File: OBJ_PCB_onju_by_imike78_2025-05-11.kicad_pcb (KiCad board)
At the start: 4 copper layers, 74.5 x 70.6 mm, 177 parts, among them J1 1775443-2, J2 TE_2345986-1, Q1 LBSS138WT1G, Q2 BC847B, SW1 CHS-01TA, U1 TPS62130, U10 SN74LVC125APWR, U11 MAX98357AETE_T, U12 FSUSB42MUX, U13 AP22802AW5-7, U2 MIC5365-1.8YC5-TR, U3 TPS62130, U4 MIC5365-0.9YC5-TR, U5 ESP32-S3R8, U6 W25Q128JVSIQ, U7 XU316-1024-QF60B-C24, U8 W25Q128JVSIQ, U9 TLV73333PDBVR, Y1 40MHz, Y2 24MHz

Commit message: production preparation
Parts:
- J2: value TE_2345986-1 -> usb_c
- R44, R7: value 49.9 -> 49.9R
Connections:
- J2 pad SH1: (no net) -> GND
- J2 pad SH2: (no net) -> GND
- J2 pad SH3: (no net) -> GND
- J2 pad SH4: (no net) -> GND
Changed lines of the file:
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@@
 		)
 		(pad_to_mask_clearance 0.03)
-		(solder_mask_min_width 0.07)
 		(allow_soldermask_bridges_in_footprints yes)
 		(tenting front back)
@@
 			)
 		)
-		(property "Value" "49.9"
+		(property "Value" "49.9R"
 			(at 0 1.43 0)
 			(layer "F.Fab")
@@
 			)
 		)
-		(property "Value" "49.9"
+		(property "Value" "49.9R"
 			(at 0 1.43 0)
 			(layer "F.Fab")
@@
 			)
 		)
-		(property "Value" "TE_2345986-1"
+		(property "Value" "usb_c"
 			(at 2.52 -6.085 37)
 			(layer "F.Fab")
@@
 			(layers "*.Cu")
 			(remove_unused_layers no)
+			(net 1 "GND")
+			(pinfunction "SHIELD")
+			(pintype "passive")
 			(thermal_bridge_angle 90)
 			(options
@@
 			(layers "*.Cu")
 			(remove_unused_layers no)
+			(net 1 "GND")
+			(pinfunction "SHIELD")
+			(pintype "passive")
 			(thermal_bridge_angle 90)
 			(options
@@
 			(layers "*.Cu" "*.Mask")
 			(remove_unused_layers no)
+			(net 1 "GND")
+			(pinfunction "SHIELD")
+			(pintype "passive")
 			(solder_mask_margin 0.102)
 		)
@@
 			(layers "*.Cu" "*.Mask")
 			(remove_unused_layers no)
+			(net 1 "GND")
+			(pinfunction "SHIELD")
+			(pintype "passive")
 			(solder_mask_margin 0.102)
 		)

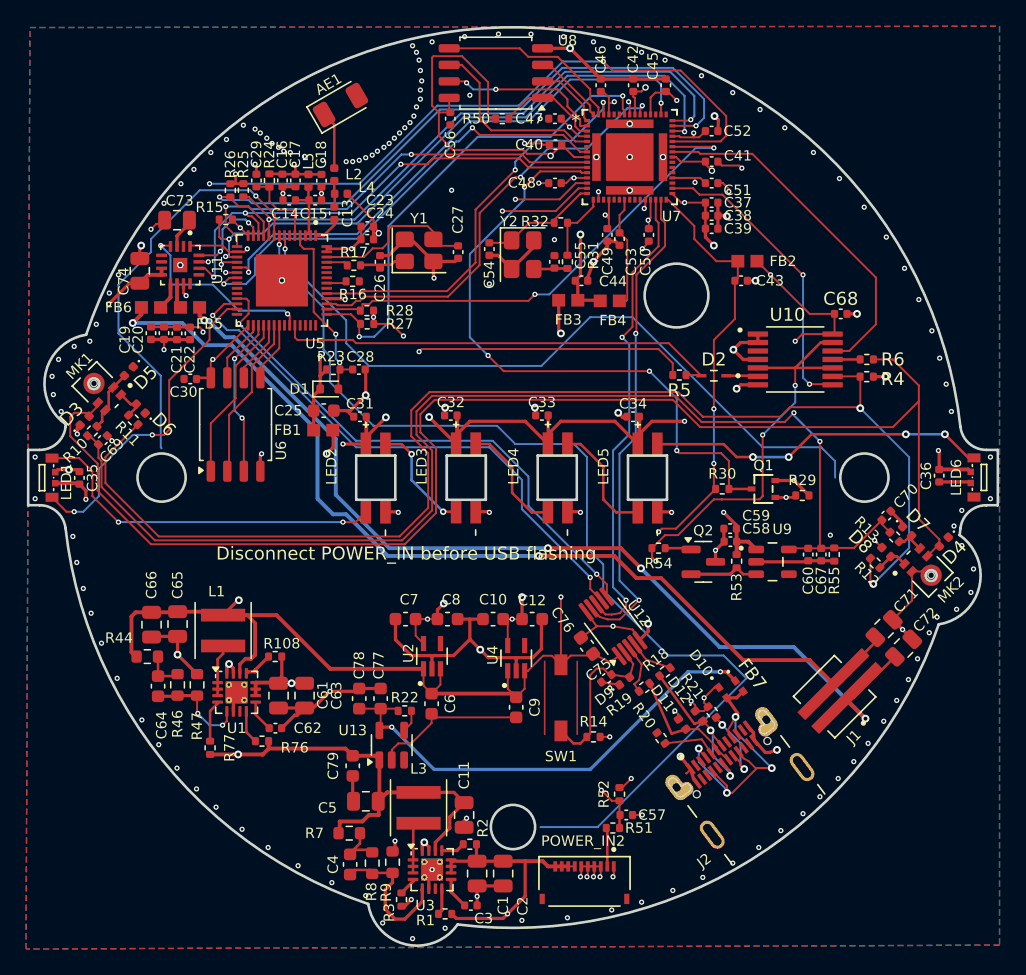
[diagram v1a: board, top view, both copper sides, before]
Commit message: final touches
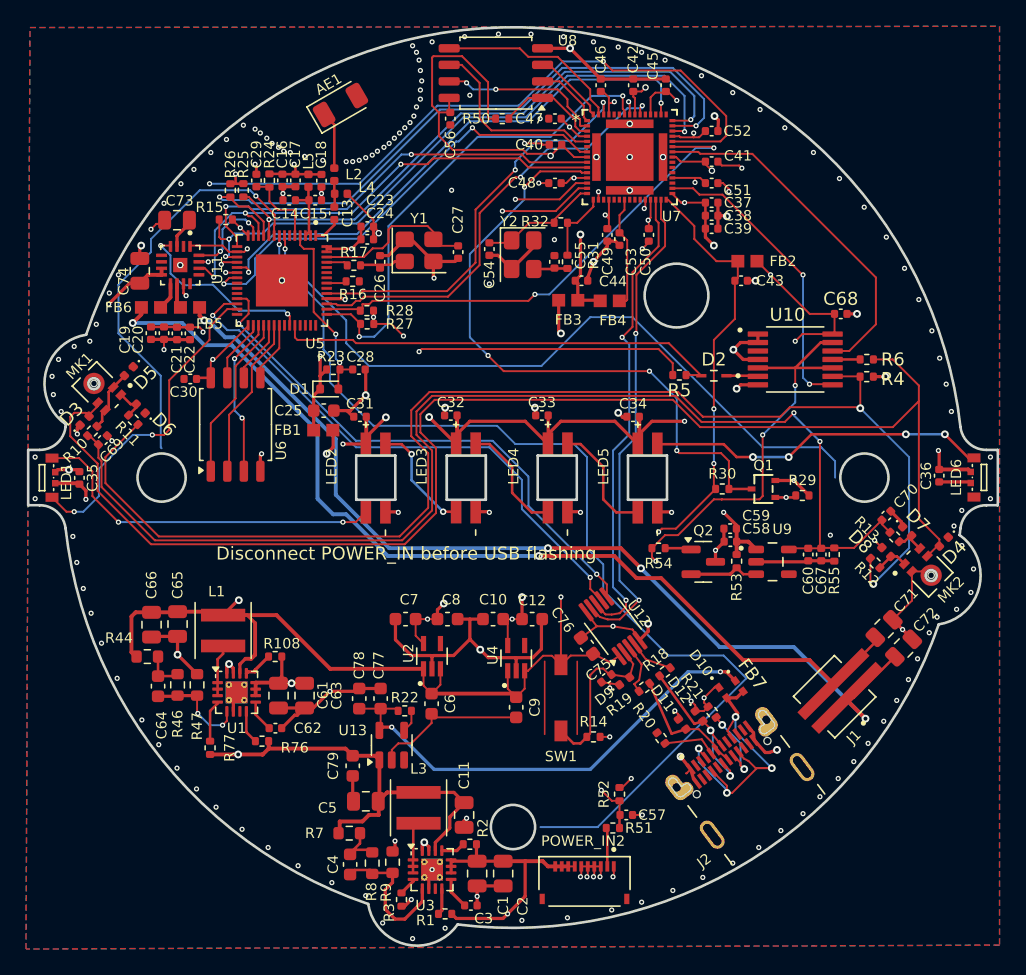
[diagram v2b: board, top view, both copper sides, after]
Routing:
- net GND: track 203.4 -> 202.8 mm
- net AUDIO_PA_EN: track 15.0 -> 14.5 mm
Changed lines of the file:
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@@
 	)
 	(segment
-		(start 154.344033 109.344033)
-		(end 154.344033 109.239039)
-		(width 0.15)
-		(layer "F.Cu")
-		(net 1)
-	)
-	(segment
 		(start 152.75 79.25)
 		(end 153.5 80)
@@
 	)
 	(segment
-		(start 102.557053 85.042947)
-		(end 102.457053 85.042947)
-		(width 0.15)
-		(layer "F.Cu")
-		(net 1)
-	)
-	(segment
 		(start 151.638907 105.201364)
 		(end 151.298636 105.201364)
@@
 	)
 	(segment
-		(start 102.771159 85.042947)
-		(end 102.814106 85)
-		(width 0.15)
-		(layer "F.Cu")
-		(net 1)
-	)
-	(segment
 		(start 109 78.46)
 		(end 109 79.25)
@@
 	)
 	(segment
-		(start 102.557053 85.042947)
-		(end 102.657053 84.942947)
-		(width 0.15)
-		(layer "F.Cu")
-		(net 1)
-	)
-	(segment
 		(start 125.100362 69.285999)
 		(end 125.100362 69.790999)
@@
 	)
 	(segment
-		(start 102.557053 85.042947)
-		(end 102.771159 85.042947)
-		(width 0.15)
-		(layer "F.Cu")
-		(net 1)
-	)
-	(segment
 		(start 148.52812 107.632662)
 		(end 148.52812 107.27812)
@@
 	)
 	(segment
+		(start 109.5 83.5)
+		(end 109 84)
+		(width 0.25)
+		(layer "In2.Cu")
+		(net 4)
+	)
+	(segment
 		(start 118.8 104.88)
 		(end 118.8 106.25)
@@
 	)
 	(segment
-		(start 109 80)
-		(end 108.25 80)
+		(start 108.25 80)
+		(end 109 80.8)
 		(width 0.25)
 		(layer "In2.Cu")
@@
 	)
 	(segment
-		(start 109 84)
-		(end 109 83.5)
-		(width 0.25)
-		(layer "In2.Cu")
-		(net 4)
-	)
-	(segment
 		(start 104.75 102.75)
 		(end 104.75 92.5)
@@
 	)
 	(segment
+		(start 116 83.5)
+		(end 109.5 83.5)
+		(width 0.25)
+		(layer "In2.Cu")
+		(net 4)
+	)
+	(segment
 		(start 126.05 84.45)
 		(end 126.8 83.7)
@@
 	)
 	(segment
-		(start 109 83.5)
-		(end 116 83.5)
-		(width 0.25)
-		(layer "In2.Cu")
-		(net 4)
-	)
-	(segment
-		(start 109 83.5)
-		(end 109 80)
+		(start 128.5 83.7)
+		(end 129.227091 84.427091)
 		(width 0.25)
 		(layer "In2.Cu")
@@
 	)
 	(segment
-		(start 128.5 83.7)
-		(end 129.227091 84.427091)
+		(start 106.25 104.25)
+		(end 104.75 102.75)
 		(width 0.25)
 		(layer "In2.Cu")
@@
 	)
 	(segment
-		(start 106.25 104.25)
-		(end 104.75 102.75)
+		(start 109 80.8)
+		(end 109 84)
 		(width 0.25)
 		(layer "In2.Cu")
@@
 	)
 	(segment
-		(start 128.761361 120.75)
-		(end 128.847862 120.663499)
-		(width 0.2)
-		(layer "F.Cu")
-		(net 16)
-	)
-	(segment
 		(start 126.75 123)
 		(end 127.5 123)
@@
 	)
 	(segment
-		(start 142.4 67.1)
-		(end 142.385113 67.114887)
-		(width 0.15)
-		(layer "F.Cu")
-		(net 22)
-	)
-	(segment
 		(start 145.985563 67.725999)
 		(end 145.985563 68.314437)
@@
 	)
 	(segment
-		(start 136.5 98.25)
-		(end 136.510362 98.260362)
-		(width 0.25)
-		(layer "F.Cu")
-		(net 23)
-	)
-	(segment
 		(start 135.060362 99.950999)
 		(end 135.410362 100.300999)
@@
 	)
 	(segment
-		(start 118.100362 65.765)
-		(end 117.729001 65.765)
-		(width 0.2)
-		(layer "F.Cu")
-		(net 28)
-	)
-	(segment
 		(start 112.595 80.155)
 		(end 112.75 80)
@@
 	)
 	(segment
-		(start 114.862182 69.887818)
-		(end 114.904534 69.93017)
-		(width 0.15)
-		(layer "B.Cu")
-		(net 35)
-	)
-	(segment
 		(start 134.5 69.1)
 		(end 119.3 69.1)
@@
 	)
 	(segment
-		(start 114.85 69.9)
-		(end 114.862182 69.887818)
-		(width 0.15)
-		(layer "In2.Cu")
-		(net 35)
-	)
-	(segment
 		(start 136.5 64.25)
 		(end 137.101049 64.851049)
@@
 	)
 	(segment
-		(start 149.416157 61.640735)
-		(end 149.479039 61.577853)
-		(width 0.15)
-		(layer "B.Cu")
-		(net 52)
-	)
-	(segment
 		(start 117.067099 69.249006)
 		(end 123.650994 69.249006)
@@
 	)
 	(segment
-		(start 113.25 67.5)
-		(end 113.27 67.52)
-		(width 0.15)
-		(layer "F.Cu")
-		(net 53)
-	)
-	(segment
 		(start 116.660362 69.410362)
 		(end 115.5 68.25)
@@
 	)
 	(segment
-		(start 114.100362 67.52)
-		(end 114.25 67.669638)
-		(width 0.15)
-		(layer "F.Cu")
-		(net 53)
-	)
-	(segment
 		(start 115.5 68.25)
 		(end 114.75 68.25)
@@
 	)
 	(segment
-		(start 109.5 74.25)
-		(end 109.5 72)
+		(start 110.5 74.3)
+		(end 109.5 73.4)
 		(width 0.15)
 		(layer "B.Cu")
@@
 	)
 	(segment
+		(start 109.5 73.4)
+		(end 109.5 72)
+		(width 0.15)
+		(layer "B.Cu")
+		(net 65)
+	)
+	(segment
 		(start 114.75 76.25)
 		(end 112.75 74.25)
@@
 	(segment
 		(start 112.75 74.25)
-		(end 109.5 74.25)
+		(end 110.5 74.3)
 		(width 0.15)
 		(layer "B.Cu")
@@
 	)
 	(segment
-		(start 124.5 86.25)
-		(end 134.25 86.25)
-		(width 0.15)
-		(layer "B.Cu")
-		(net 75)
-	)
-	(segment
 		(start 137 89)
 		(end 137 91.25)
@@
 	(segment
 		(start 123.75 86.25)
-		(end 124.5 86.25)
+		(end 134.25 86.25)
 		(width 0.15)
 		(layer "B.Cu")
@@
 	)
 	(segment
-		(start 139.560362 63.5)
-		(end 139.689221 63.5)
-		(width 0.2)
-		(layer "F.Cu")
-		(net 91)
-	)
-	(segment
 		(start 131.9 56.7)
 		(end 133.9 58.7)
@@
 	)
 	(segment
-		(start 147.25 69.25)
-		(end 147.5 69.5)
-		(width 0.15)
-		(layer "F.Cu")
-		(net 115)
-	)
-	(segment
 		(start 147.5 69.5)
 		(end 147.5 71.3)
@@
 	(segment
 		(start 147.185713 69.185713)
-		(end 147.25 69.25)
+		(end 147.5 69.5)
 		(width 0.15)
 		(layer "F.Cu")
@@
 		(net 118)
 	)
-	(segment
-		(start 103.129376 85.860624)
-		(end 103.129376 86.089376)
-		(width 0.2)
-		(layer "F.Cu")
-		(net 118)
-	)
 	(via
 		(at 159.4 86.3)
@@
 	)
 	(segment
-		(start 145.7 96.8)
+		(start 145.3 96.8)
 		(end 147.2 96.8)
 		(width 0.3)
@@
 		(net 132)
 	)
-	(segment
-		(start 145.3 96.8)
-		(end 145.7 96.8)
-		(width 0.3)
-		(layer "F.Cu")
-		(net 132)
-	)
 	(via
 		(at 137.8 95.1)
@@
 	)
 	(segment
-		(start 161.4 106)
-		(end 161.5 106)
-		(width 0.15)
-		(layer "F.Cu")
-		(net 133)
-	)
-	(segment
 		(start 161.5 106.2)
 		(end 161.5 106)
@@
 	(segment
 		(start 151.7 102.1)
-		(end 152.9 102.1)
+		(end 157.4 102.1)
 		(width 0.3)
 		(layer "B.Cu")
@@
 		(width 0.3)
 		(layer "B.Cu")
-		(net 133)
-	)
-	(segment
-		(start 152.9 102.1)
-		(end 157.4 102.1)
-		(width 0.3)
-		(layer "B.Cu")

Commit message: final touches
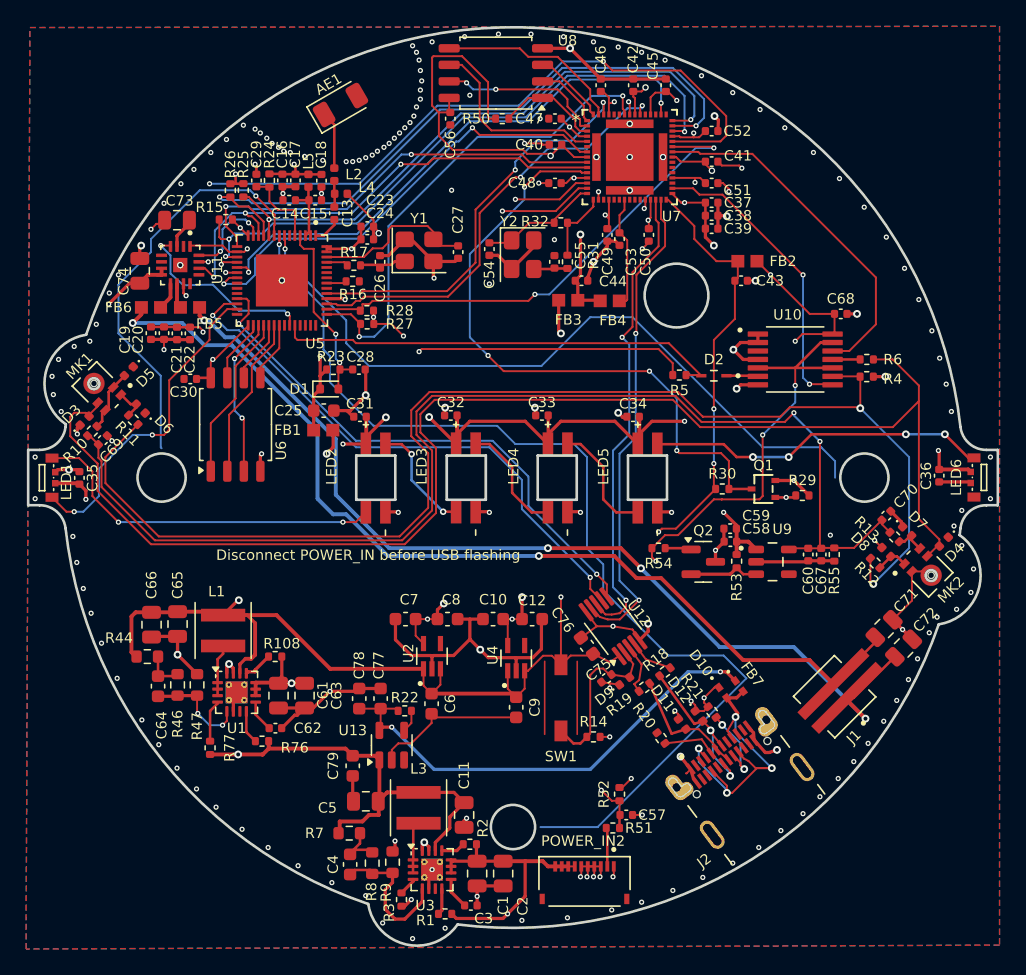
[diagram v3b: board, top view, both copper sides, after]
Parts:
- C31, C32, C33, C34, C35, C36: value 0.1uF -> 100nF
- D11, D12, D3, D4, D5, D6, D7, D8, D9: value PESD0402-050 -> PESD0402V05
- SW1: value CHS-01TA -> SMXS‑01K‑TP
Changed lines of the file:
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@@
 			)
 		)
-		(property "Value" "0.1uF"
+		(property "Value" "100nF"
 			(at 0 1.16 90)
 			(layer "F.Fab")
@@
 			(effects
 				(font
-					(size 1 1)
-					(thickness 0.15)
+					(size 0.8 0.8)
+					(thickness 0.12)
 				)
 			)
 		)
-		(property "Value" "PESD0402-050"
+		(property "Value" "PESD0402V05"
 			(at 0 1.17 45)
 			(layer "F.Fab")
@@
 			)
 		)
-		(property "Description" "PESD0402-050, 5V TVS, 0.3pF"
+		(property "Description" "PESD0402V05, 5V TVS, 0.3pF"
 			(at 0 0 45)
 			(layer "F.Fab")
@@
 			(effects
 				(font
-					(size 1 1)
-					(thickness 0.15)
+					(size 0.8 0.8)
+					(thickness 0.12)
 				)
 			)
 		)
-		(property "Value" "PESD0402-050"
+		(property "Value" "PESD0402V05"
 			(at 0 1.17 135)
 			(layer "F.Fab")
@@
 			)
 		)
-		(property "Description" "PESD0402-050, 5V TVS, 0.3pF"
+		(property "Description" "PESD0402V05, 5V TVS, 0.3pF"
 			(at 0 0 135)
 			(layer "F.Fab")
@@
 			(effects
 				(font
-					(size 1 1)
-					(thickness 0.15)
+					(size 0.8 0.8)
+					(thickness 0.12)
 				)
 			)
 		)
-		(property "Value" "PESD0402-050"
+		(property "Value" "PESD0402V05"
 			(at 0 1.17 135)
 			(layer "F.Fab")
@@
 			)
 		)
-		(property "Description" "PESD0402-050, 5V TVS, 0.3pF"
+		(property "Description" "PESD0402V05, 5V TVS, 0.3pF"
 			(at 0 0 135)
 			(layer "F.Fab")
@@
 			)
 		)
-		(property "Value" "CHS-01TA"
+		(property "Value" "SMXS‑01K‑TP"
 			(at 0.839974 4.253187 0)
 			(layer "Dwgs.User")
@@
 			)
 		)
-		(property "MF" "Nidec Copal"
+		(property "MF" "SM Switch"
 			(at 0 0 0)
 			(unlocked yes)
@@
 			)
 		)
-		(property "Package" "None"
-			(at 0 0 0)
-			(unlocked yes)
-			(layer "F.Fab")
-			(hide yes)
-			(effects
-				(font
-					(size 1 1)
-					(thickness 0.15)
-				)
-			)
-		)
-		(property "Price" "None"
-			(at 0 0 0)
-			(unlocked yes)
-			(layer "F.Fab")
-			(hide yes)
-			(effects
-				(font
-					(size 1 1)
-					(thickness 0.15)
-				)
-			)
-		)
-		(property "SnapEDA_Link" "https://www.snapeda.com/parts/CHS-01TA/Nidec/view-part/?ref=snap"
-			(at 0 0 0)
-			(unlocked yes)
-			(layer "F.Fab")
-			(hide yes)
-			(effects
-				(font
-					(size 1 1)
-					(thickness 0.15)
-				)
-			)
-		)
-		(property "MP" "CHS-01TA"
-			(at 0 0 0)
-			(unlocked yes)
-			(layer "F.Fab")
-			(hide yes)
-			(effects
-				(font
-					(size 1 1)
-					(thickness 0.15)
-				)
-			)
-		)
-		(property "Availability" "In Stock"
-			(at 0 0 0)
-			(unlocked yes)
-			(layer "F.Fab")
-			(hide yes)
-			(effects
-				(font
-					(size 1 1)
-					(thickness 0.15)
-				)
-			)
-		)
-		(property "Check_prices" "https://www.snapeda.com/parts/CHS-01TA/Nidec/view-part/?ref=eda"
+		(property "MP" "SMXS‑01K‑TP"
 			(at 0 0 0)
 			(unlocked yes)
@@
 			(effects
 				(font
-					(size 1 1)
-					(thickness 0.15)
+					(size 0.8 0.8)
+					(thickness 0.12)
 				)
 			)
@@
 			(effects
 				(font
-					(size 1 1)
-					(thickness 0.15)
+					(size 0.8 0.8)
+					(thickness 0.12)
 				)
 			)
@@
 			)
 		)
-		(property "Value" "PESD0402-050"
+		(property "Value" "PESD0402V05"
 			(at 0 1.170001 127)
 			(layer "F.Fab")
@@
 			)
 		)
-		(property "Description" "PESD0402-050, 5V TVS, 0.3pF"
+		(property "Description" "PESD0402V05, 5V TVS, 0.3pF"
 			(at 0 0 127)
 			(layer "F.Fab")
@@
 			)
 		)
-		(property "Function" "MIC"
+		(property "Function" "USB"
 			(at 0 0 307)
 			(unlocked yes)
@@
 			(effects
 				(font
-					(size 1 1)
-					(thickness 0.15)
+					(size 0.8 0.8)
+					(thickness 0.12)
 				)
 			)
@@
 			)
 		)
-		(property "Value" "PESD0402-050"
+		(property "Value" "PESD0402V05"
 			(at 0 1.170001 37)
 			(layer "F.Fab")
@@
 			)
 		)
-		(property "Description" "PESD0402-050, 5V TVS, 0.3pF"
+		(property "Description" "PESD0402V05, 5V TVS, 0.3pF"
 			(at 0 0 37)
 			(layer "F.Fab")
@@
 			)
 		)
-		(property "Function" "MIC"
+		(property "Function" "USB"
 			(at 0 0 37)
 			(unlocked yes)
@@
 			)
 		)
-		(property "Value" "0.1uF"
+		(property "Value" "100nF"
 			(at 0 1.16 0)
 			(layer "F.Fab")
@@
 			)
 		)
-		(property "Value" "0.1uF"
+		(property "Value" "100nF"
 			(at 0 1.16 0)
 			(layer "F.Fab")
@@
 			)
 		)
-		(property "Value" "0.1uF"
+		(property "Value" "100nF"
 			(at 0 1.16 90)
 			(layer "F.Fab")
@@
 			(effects
 				(font
-					(size 1 1)
-					(thickness 0.15)
+					(size 0.8 0.8)
+					(thickness 0.12)
 				)
 			)
 		)
-		(property "Value" "PESD0402-050"
+		(property "Value" "PESD0402V05"
 			(at 0 1.17 45)
 			(layer "F.Fab")
@@
 			)
 		)
-		(property "Description" "PESD0402-050, 5V TVS, 0.3pF"
+		(property "Description" "PESD0402V05, 5V TVS, 0.3pF"
 			(at 0 0 45)
 			(layer "F.Fab")
@@
 			(effects
 				(font
-					(size 1 1)
-					(thickness 0.15)
+					(size 0.8 0.8)
+					(thickness 0.12)
 				)
 			)
@@
 			(effects
 				(font
-					(size 1 1)
-					(thickness 0.15)
+					(size 0.8 0.8)
+					(thickness 0.12)
 				)
 			)
 		)
-		(property "Value" "PESD0402-050"
+		(property "Value" "PESD0402V05"
 			(at 0 1.17 135)
 			(layer "F.Fab")
@@
 			)
 		)
-		(property "Description" "PESD0402-050, 5V TVS, 0.3pF"
+		(property "Description" "PESD0402V05, 5V TVS, 0.3pF"
 			(at 0 0 135)
 			(layer "F.Fab")
@@
 			(effects
 				(font
-					(size 1 1)
-					(thickness 0.15)
+					(size 0.8 0.8)
+					(thickness 0.12)
 				)
 			)
@@
 			)
 		)
-		(property "Value" "0.1uF"
+		(property "Value" "100nF"
 			(at 0 1.16 0)
 			(layer "F.Fab")
@@
 			(effects
 				(font
-					(size 1 1)
-					(thickness 0.15)
+					(size 0.8 0.8)
+					(thickness 0.12)
 				)
 			)
 		)
-		(property "Value" "PESD0402-050"
+		(property "Value" "PESD0402V05"
 			(at 0 1.17 45)
 			(layer "F.Fab")
@@
 			)
 		)
-		(property "Description" "PESD0402-050, 5V TVS, 0.3pF"
+		(property "Description" "PESD0402V05, 5V TVS, 0.3pF"
 			(at 0 0 45)
 			(layer "F.Fab")
@@
 			)
 		)
-		(property "Description" ""
+		(property "Description" "2345986-1"
 			(at 0 0 37)
 			(layer "F.Fab")
@@
 		)
 		(embedded_fonts no)
+		(model "D:/temp/Onju voice/Parts/usb_c.step"
+			(offset
+				(xyz 0 -4 1.5)
+			)
+			(scale
+				(xyz 1 1 1)
+			)
+			(rotate
+				(xyz -90 -0 -0)
+			)
+		)
 	)
 	(footprint "Onju:SOP65P640X120-14N"
@@
 			(effects
 				(font
-					(size 1 1)
-					(thickness 0.15)
+					(size 0.8 0.8)
+					(thickness 0.12)
 				)
 			)
@@
 		)
 		(embedded_fonts no)
+		(model "D:/temp/Onju voice/Parts/DMM-3526-B-R.step"
+			(offset
+				(xyz 0 0 0.4)
+			)
+			(scale
+				(xyz 1 1 1)
+			)
+			(rotate
+				(xyz -90 -0 -0)
+			)
+		)
 	)
 	(footprint "Resistor_SMD:R_0402_1005Metric"
@@
 			(effects
 				(font
-					(size 1 1)
-					(thickness 0.15)
+					(size 0.8 0.8)
+					(thickness 0.12)
 				)
 			)
@@
 			)
 		)
-		(property "Value" "0.1uF"
+		(property "Value" "100nF"
 			(at 0 1.16 0)
 			(layer "F.Fab")
@@
 			)
 		)
-		(property "Value" "PESD0402-050"
+		(property "Value" "PESD0402V05"
 			(at 0 1.170001 127)
 			(layer "F.Fab")
@@
 			)
 		)
-		(property "Description" "PESD0402-050, 5V TVS, 0.3pF"
+		(property "Description" "PESD0402V05, 5V TVS, 0.3pF"
 			(at 0 0 127)
 			(layer "F.Fab")
@@
 			)
 		)
-		(property "Function" "MIC"
+		(property "Function" "USB"
 			(at 0 0 307)
 			(unlocked yes)
@@
 		(effects
 			(font
-				(size 1 1)
-				(thickness 0.125)
+				(size 0.8 0.8)
+				(thickness 0.12)
 			)
 			(justify left bottom)
